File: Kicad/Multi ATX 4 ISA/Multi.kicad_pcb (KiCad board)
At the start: 2 copper layers, 121.9 x 172.7 mm, 89 parts, among them J1 Bus_ISA_8bit, J10 Conn_02x08_Counter_Clockwise, J2 Mini-DIN-6, J3 SPK, J6 PWR ON, J7 Bus_ISA_8bit, J8 Bus_ISA_8bit, J9 Bus_ISA_8bit, SW1 RESET, U1 74LS139, U11 8284, U117 74LS139, U12 74LS138, U13 74LS138, U14 74LS74, U15 74LS573, U16 74LS04, U17 74LS139, U19 82C42/83C42, U2 74LS245, U20 74LS07, U3 33 ohm, U9 74LS138, Y2 14.31818 MHz

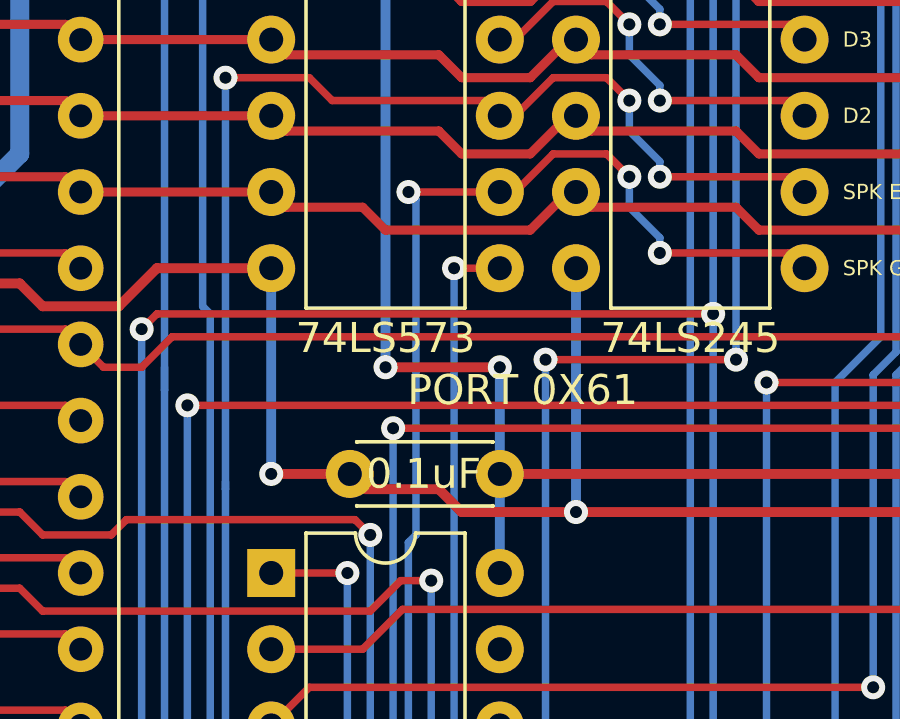
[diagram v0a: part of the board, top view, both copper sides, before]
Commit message: 4 Slot Main board update
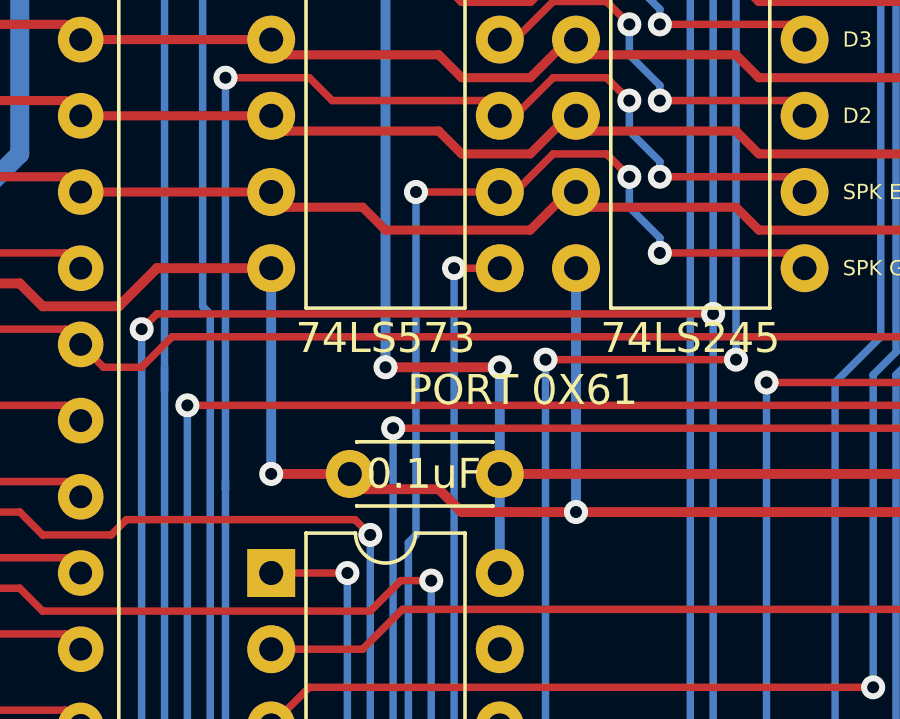
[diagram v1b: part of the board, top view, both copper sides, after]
